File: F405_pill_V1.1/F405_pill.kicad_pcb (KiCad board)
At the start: 4 copper layers, 53.8 x 19.4 mm, 50 parts, among them J1 Conn_01x04_Male, J2 Conn_01x04_Male, J4 TYPE-C-31-M-12, U1 STM32F405RGTx, U2 MAX3051EKA+T, U3 LM1117-3.3, U4 STM32F405_pill, U5 HT7550-1, Y1 Crystal_GND24

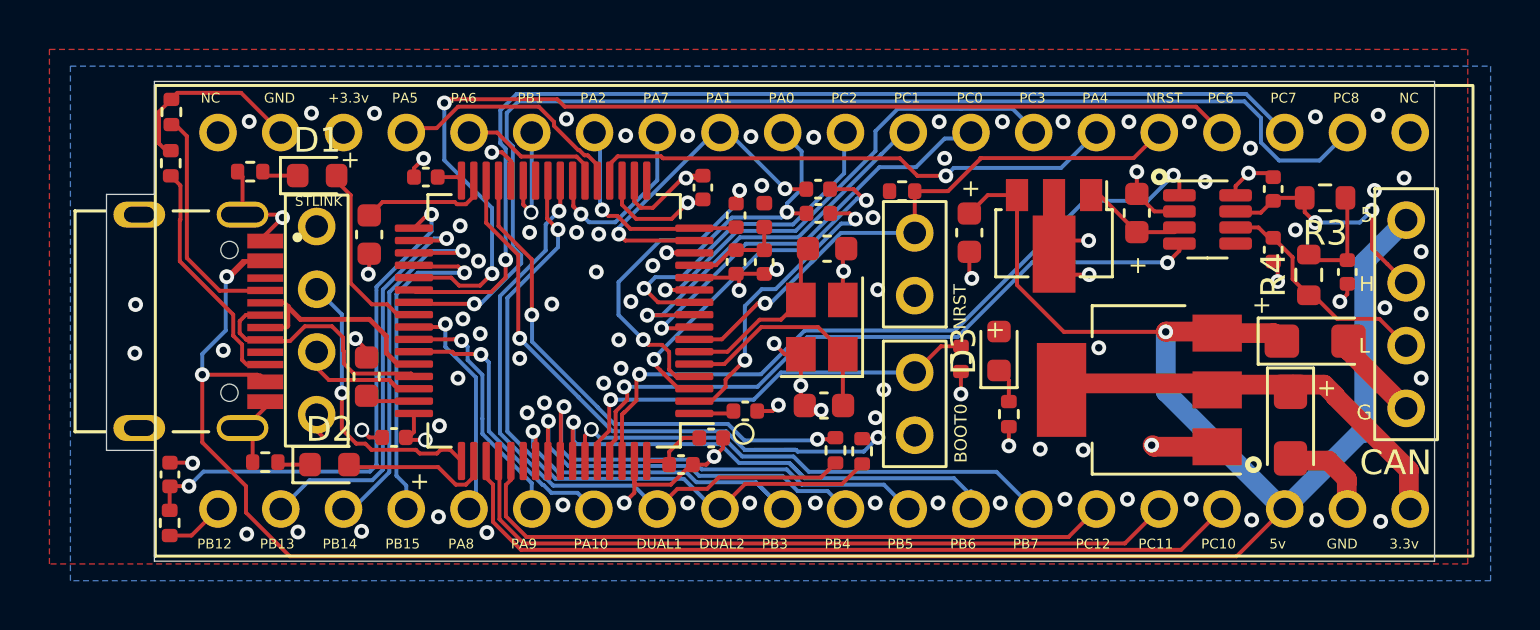
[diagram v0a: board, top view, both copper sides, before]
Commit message: minor edits
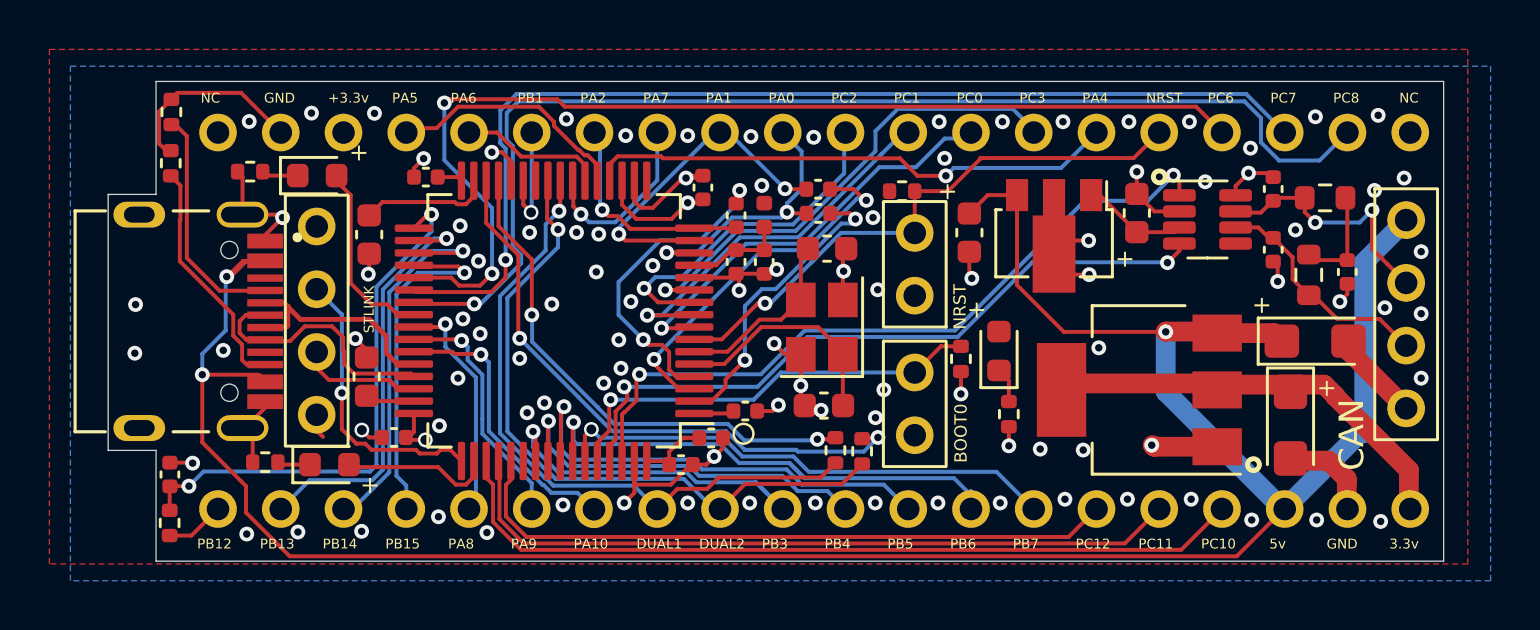
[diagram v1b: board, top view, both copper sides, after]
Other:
- board size 53.8 x 19.4 mm -> 54.1 x 19.4 mm
- board text removed: "5"
- board text removed: "G"
- board text removed: "H"
- board text removed: "L"
